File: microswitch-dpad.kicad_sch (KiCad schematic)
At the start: 12 parts, among them J1 Conn_01x05_Socket, J2 Conn_01x03_Socket, U1 D2LS-21_C3823622, U2 D2LS-21_C3823622, U3 D2LS-21_C3823622, U4 D2LS-21_C3823622

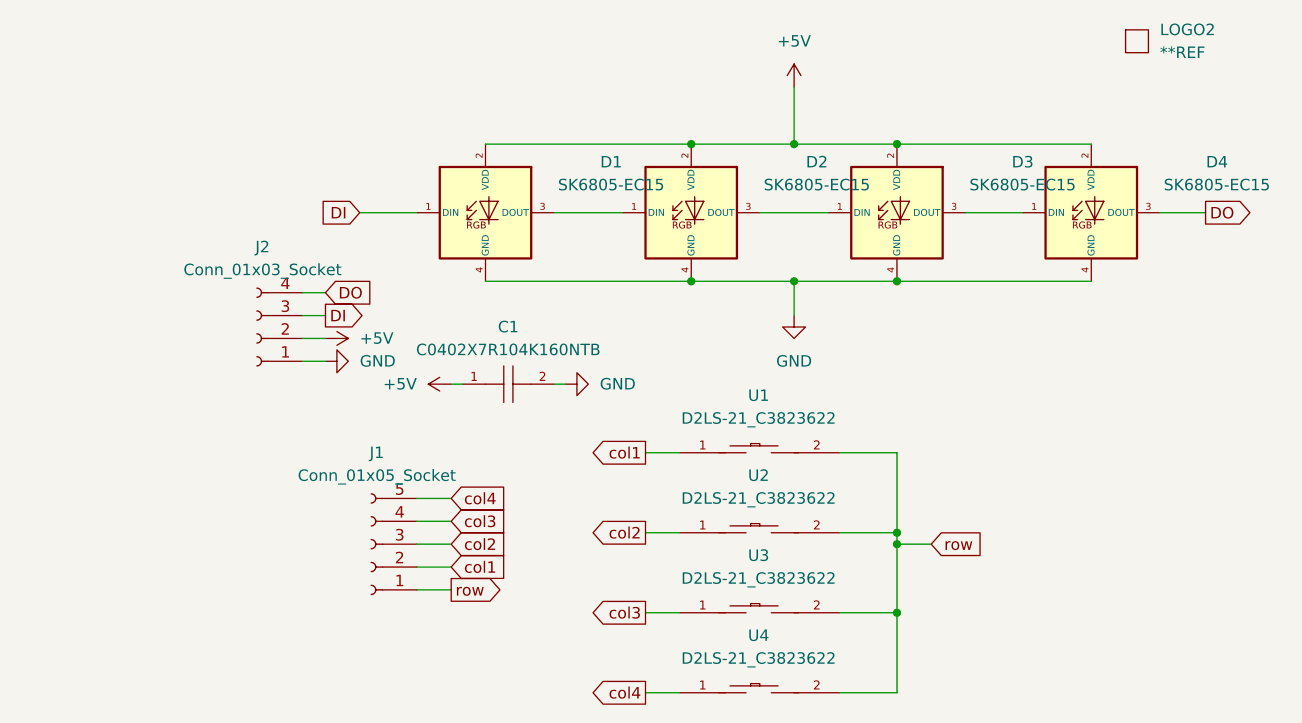
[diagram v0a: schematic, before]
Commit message: production submitted
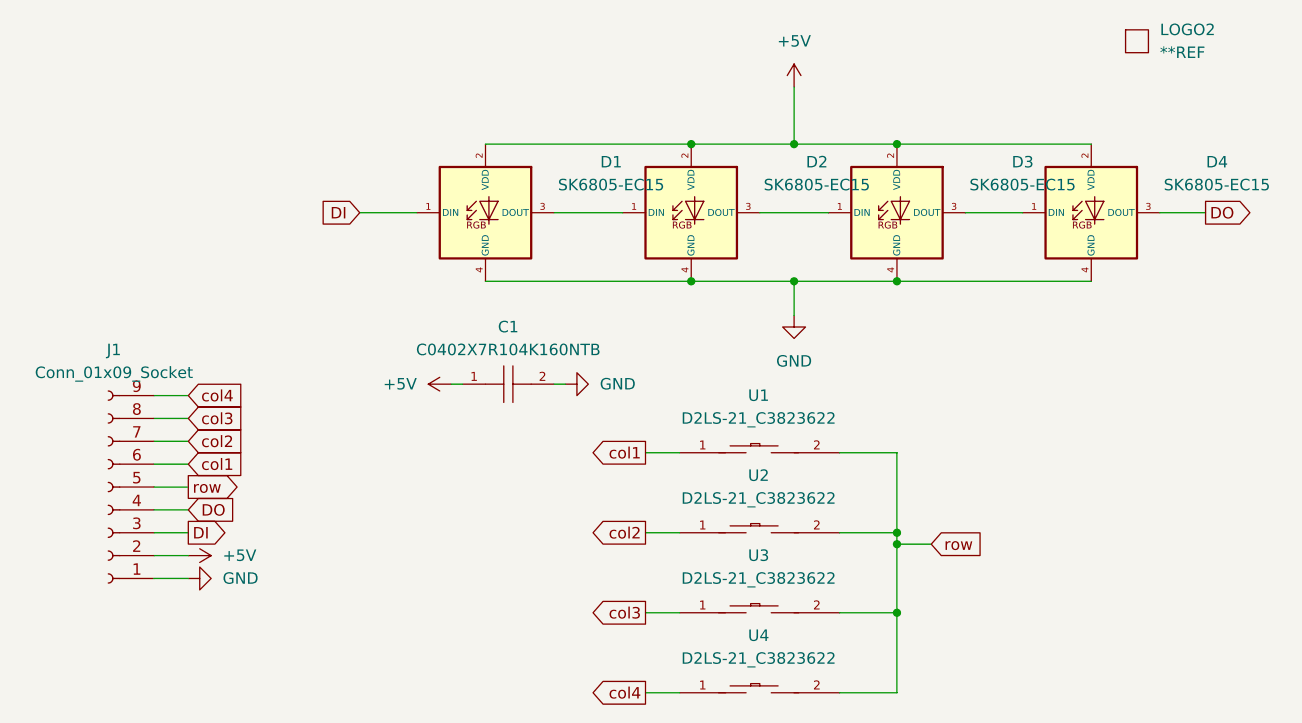
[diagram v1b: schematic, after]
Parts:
- removed J1: Conn_01x05_Socket, Connector_PinSocket_2.54mm:PinSocket_1x05_P2.54mm_Vertical, symbol Connector:Conn_01x05_Socket
- removed J2: Conn_01x03_Socket, Connector_PinSocket_2.54mm:PinSocket_1x04_P2.54mm_Vertical, symbol Connector:Conn_01x04_Socket
- added J1: Conn_01x09_Socket, Connector_PinSocket_1.27mm:PinSocket_1x09_P1.27mm_Vertical, symbol Connector:Conn_01x09_Socket
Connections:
- net +5V: now also J1.2 (Pin_2)
- net DI: now also J1.3 (Pin_3)
- net DO: now also J1.4 (Pin_4)
- net GND: now also J1.1 (Pin_1)
- net col1: now also J1.6 (Pin_6)
- net col2: now also J1.7 (Pin_7)
- net col3: now also J1.8 (Pin_8)
- net col4: now also J1.9 (Pin_9)
- net row: now also J1.5 (Pin_5)
